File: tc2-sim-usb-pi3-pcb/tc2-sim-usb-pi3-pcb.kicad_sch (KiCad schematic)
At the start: 5 parts, among them J11 Conn_01x08, J2 Conn_01x03

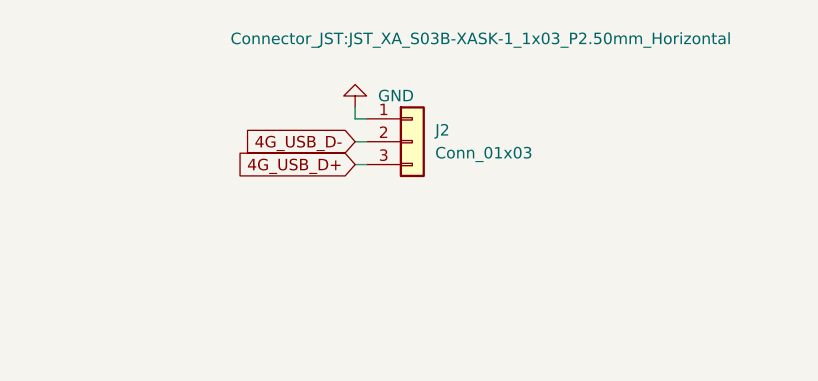
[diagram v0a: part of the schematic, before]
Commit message: v0.4.0
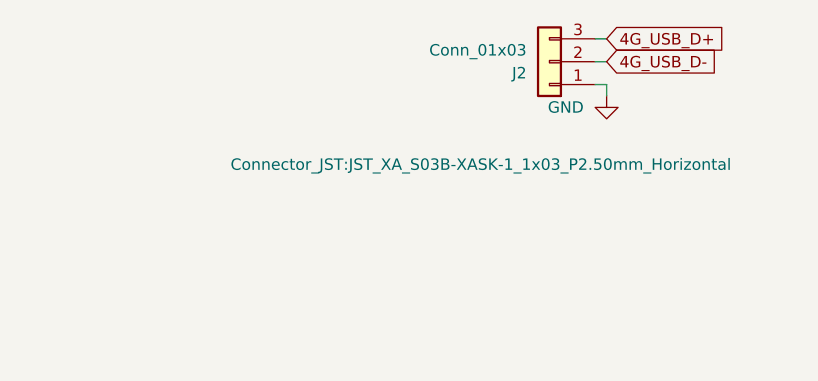
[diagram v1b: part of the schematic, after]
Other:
- moved on the sheet: J2
